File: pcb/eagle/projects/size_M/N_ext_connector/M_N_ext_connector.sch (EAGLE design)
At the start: 16 parts

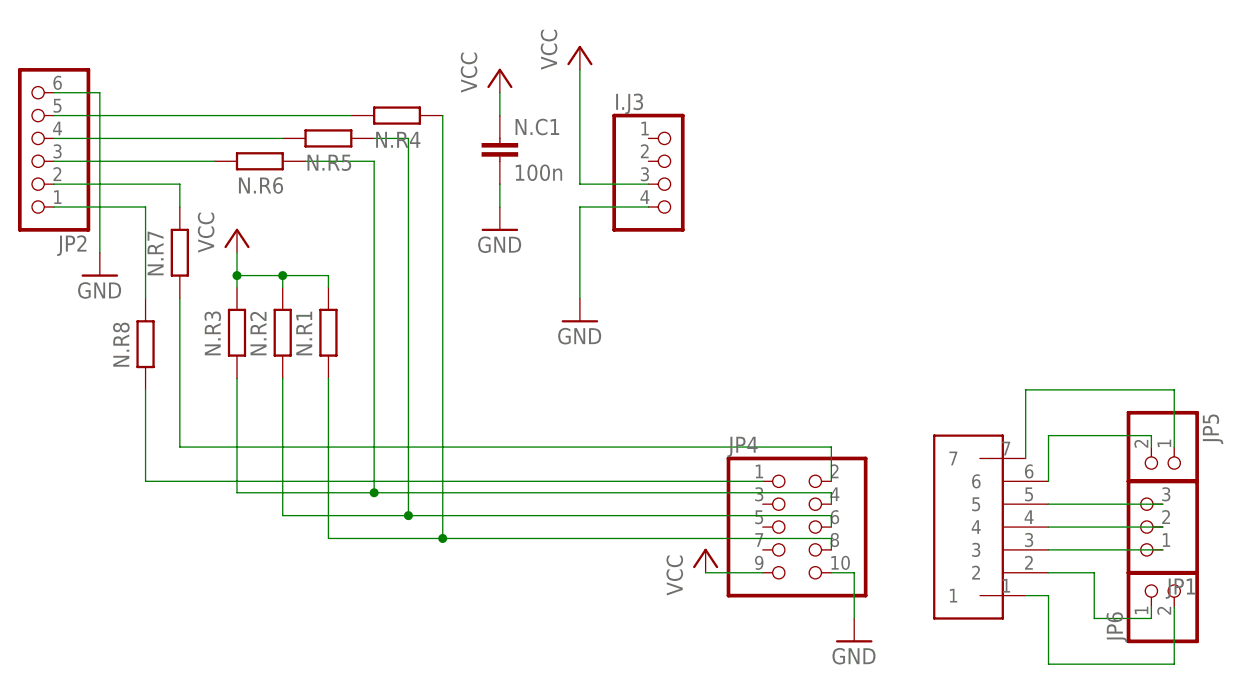
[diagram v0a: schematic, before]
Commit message: just adjustments
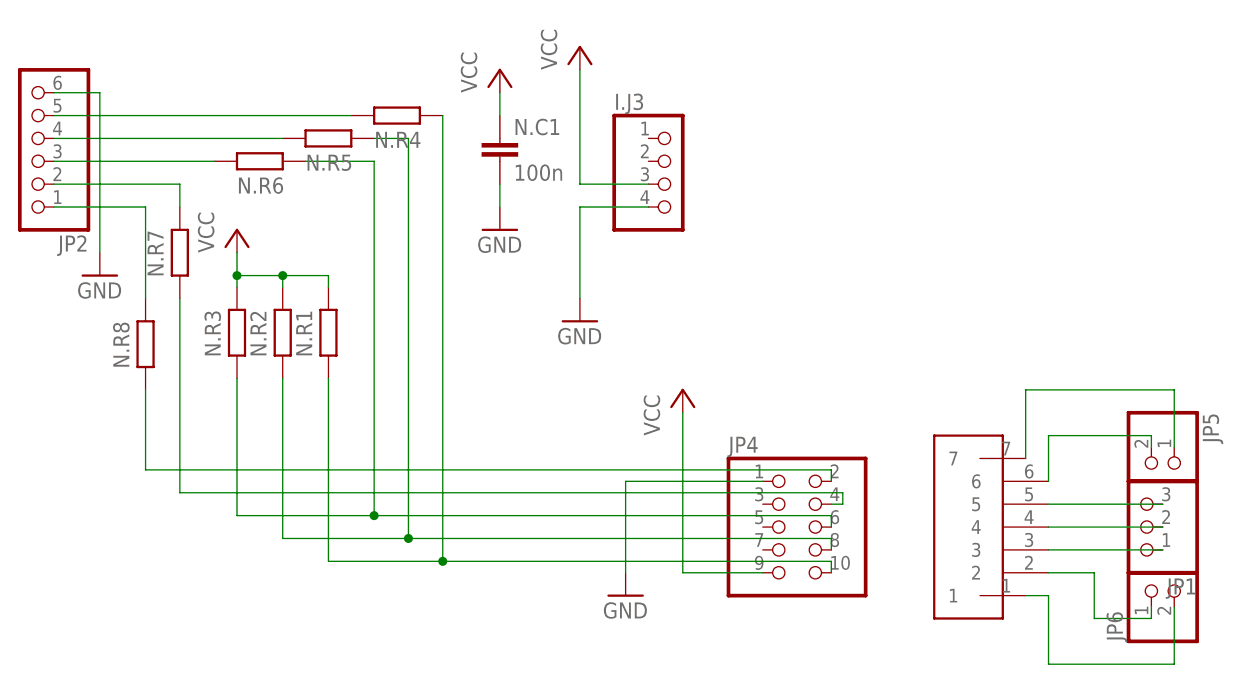
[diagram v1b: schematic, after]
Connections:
- net N$1 renamed PA6
- net N$12 renamed PA7
- net N$13 renamed SDA1
- net N$14 renamed PA3
- removed net N$15: JP6.2, U$1.1
- new net SCL1: JP5.2, U$1.6
- net GND: now also JP4.1; no longer JP4.10
- net GND1: now also JP5.1, U$1.7; no longer JP5.2, U$1.6
- net N$10: now also JP4.4; no longer JP4.2
- net N$11: now also JP4.2; no longer JP4.1
- net N$2: now also JP4.10; no longer JP4.8
- net N$3: now also JP4.8; no longer JP4.6
- net N$9: now also JP4.6; no longer JP4.4
- net VCC1: now also JP6.2, U$1.1; no longer JP5.1, U$1.7
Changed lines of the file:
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@@
 <attribute name="VALUE" x="111.76" y="20.32" size="1.778" layer="96"/>
 </instance>
-<instance part="GND4" gate="1" x="144.78" y="-12.7" smashed="yes">
-<attribute name="VALUE" x="142.24" y="-15.24" size="1.778" layer="96"/>
+<instance part="GND4" gate="1" x="119.38" y="-7.62" smashed="yes">
+<attribute name="VALUE" x="116.84" y="-10.16" size="1.778" layer="96"/>
 </instance>
 <instance part="GND5" gate="1" x="60.96" y="27.94" smashed="yes">
 <attribute name="VALUE" x="58.42" y="25.4" size="1.778" layer="96"/>
 </instance>
-<instance part="P+4" gate="VCC" x="128.27" y="-2.54" smashed="yes">
-<attribute name="VALUE" x="125.73" y="-7.62" size="1.778" layer="96" rot="R90"/>
+<instance part="P+4" gate="VCC" x="125.73" y="15.24" smashed="yes">
+<attribute name="VALUE" x="123.19" y="10.16" size="1.778" layer="96" rot="R90"/>
 </instance>
 <instance part="P+3" gate="VCC" x="76.2" y="33.02" smashed="yes">
@@
 <segment>
 <pinref part="GND4" gate="1" pin="GND"/>
-<wire x1="142.24" y1="-5.08" x2="144.78" y2="-5.08" width="0.1524" layer="91"/>
-<wire x1="144.78" y1="-5.08" x2="144.78" y2="-10.16" width="0.1524" layer="91"/>
-<pinref part="JP4" gate="A" pin="10"/>
+<pinref part="JP4" gate="A" pin="1"/>
+<wire x1="119.38" y1="-5.08" x2="119.38" y2="5.08" width="0.1524" layer="91"/>
+<wire x1="119.38" y1="5.08" x2="134.62" y2="5.08" width="0.1524" layer="91"/>
 </segment>
 </net>
@@
 <segment>
 <pinref part="P+4" gate="VCC" pin="VCC"/>
-<wire x1="128.27" y1="-5.08" x2="134.62" y2="-5.08" width="0.1524" layer="91"/>
 <pinref part="JP4" gate="A" pin="9"/>
+<wire x1="125.73" y1="12.7" x2="125.73" y2="-5.08" width="0.1524" layer="91"/>
+<wire x1="125.73" y1="-5.08" x2="134.62" y2="-5.08" width="0.1524" layer="91"/>
 </segment>
 </net>
 <net name="N$2" class="0">
 <segment>
-<wire x1="86.36" y1="-1.27" x2="99.06" y2="-1.27" width="0.1524" layer="91"/>
+<wire x1="86.36" y1="-3.81" x2="99.06" y2="-3.81" width="0.1524" layer="91"/>
 <pinref part="N.R1" gate="G$1" pin="2"/>
-<wire x1="86.36" y1="16.51" x2="86.36" y2="-1.27" width="0.1524" layer="91"/>
-<wire x1="99.06" y1="-1.27" x2="99.06" y2="45.72" width="0.1524" layer="91"/>
+<wire x1="86.36" y1="16.51" x2="86.36" y2="-3.81" width="0.1524" layer="91"/>
+<wire x1="99.06" y1="-3.81" x2="99.06" y2="45.72" width="0.1524" layer="91"/>
 <pinref part="N.R4" gate="G$1" pin="2"/>
+<wire x1="99.06" y1="-3.81" x2="142.24" y2="-3.81" width="0.1524" layer="91"/>
+<junction x="99.06" y="-3.81"/>
+<pinref part="JP4" gate="A" pin="10"/>
+<wire x1="142.24" y1="-5.08" x2="142.24" y2="-3.81" width="0.1524" layer="91"/>
+</segment>
+</net>
+<net name="N$3" class="0">
+<segment>
+<wire x1="81.28" y1="-1.27" x2="95.25" y2="-1.27" width="0.1524" layer="91"/>
+<pinref part="N.R2" gate="G$1" pin="2"/>
+<wire x1="81.28" y1="16.51" x2="81.28" y2="-1.27" width="0.1524" layer="91"/>
+<wire x1="91.44" y1="43.18" x2="95.25" y2="43.18" width="0.1524" layer="91"/>
+<wire x1="95.25" y1="43.18" x2="95.25" y2="-1.27" width="0.1524" layer="91"/>
+<pinref part="N.R5" gate="G$1" pin="2"/>
+<wire x1="95.25" y1="-1.27" x2="142.24" y2="-1.27" width="0.1524" layer="91"/>
+<junction x="95.25" y="-1.27"/>
 <pinref part="JP4" gate="A" pin="8"/>
-<wire x1="99.06" y1="-1.27" x2="142.24" y2="-1.27" width="0.1524" layer="91"/>
-<wire x1="142.24" y1="-1.27" x2="142.24" y2="-2.54" width="0.1524" layer="91"/>
-<junction x="99.06" y="-1.27"/>
-</segment>
-</net>
-<net name="N$3" class="0">
-<segment>
-<wire x1="81.28" y1="1.27" x2="95.25" y2="1.27" width="0.1524" layer="91"/>
-<pinref part="N.R2" gate="G$1" pin="2"/>
-<wire x1="81.28" y1="16.51" x2="81.28" y2="1.27" width="0.1524" layer="91"/>
-<wire x1="91.44" y1="43.18" x2="95.25" y2="43.18" width="0.1524" layer="91"/>
-<wire x1="95.25" y1="43.18" x2="95.25" y2="1.27" width="0.1524" layer="91"/>
-<pinref part="N.R5" gate="G$1" pin="2"/>
-<pinref part="JP4" gate="A" pin="6"/>
-<wire x1="95.25" y1="1.27" x2="142.24" y2="1.27" width="0.1524" layer="91"/>
-<wire x1="142.24" y1="1.27" x2="142.24" y2="0" width="0.1524" layer="91"/>
-<junction x="95.25" y="1.27"/>
+<wire x1="142.24" y1="-2.54" x2="142.24" y2="-1.27" width="0.1524" layer="91"/>
 </segment>
 </net>
 <net name="N$10" class="0">
 <segment>
-<wire x1="69.85" y1="25.4" x2="69.85" y2="8.89" width="0.1524" layer="91"/>
+<wire x1="69.85" y1="25.4" x2="69.85" y2="3.81" width="0.1524" layer="91"/>
 <pinref part="N.R7" gate="G$1" pin="2"/>
-<pinref part="JP4" gate="A" pin="2"/>
-<wire x1="142.24" y1="5.08" x2="142.24" y2="8.89" width="0.1524" layer="91"/>
-<wire x1="142.24" y1="8.89" x2="69.85" y2="8.89" width="0.1524" layer="91"/>
+<wire x1="143.51" y1="3.81" x2="69.85" y2="3.81" width="0.1524" layer="91"/>
+<pinref part="JP4" gate="A" pin="4"/>
+<wire x1="142.24" y1="2.54" x2="143.51" y2="2.54" width="0.1524" layer="91"/>
+<wire x1="143.51" y1="2.54" x2="143.51" y2="3.81" width="0.1524" layer="91"/>
 </segment>
 </net>
@@
 <net name="N$11" class="0">
 <segment>
-<pinref part="JP4" gate="A" pin="1"/>
-<wire x1="66.04" y1="15.24" x2="66.04" y2="5.08" width="0.1524" layer="91"/>
 <pinref part="N.R8" gate="G$1" pin="2"/>
-<wire x1="134.62" y1="5.08" x2="66.04" y2="5.08" width="0.1524" layer="91"/>
+<wire x1="66.04" y1="15.24" x2="66.04" y2="6.35" width="0.1524" layer="91"/>
+<pinref part="JP4" gate="A" pin="2"/>
+<wire x1="142.24" y1="5.08" x2="142.24" y2="6.35" width="0.1524" layer="91"/>
+<wire x1="142.24" y1="6.35" x2="66.04" y2="6.35" width="0.1524" layer="91"/>
 </segment>
 </net>
 <net name="N$9" class="0">
 <segment>
-<pinref part="JP4" gate="A" pin="4"/>
-<wire x1="142.24" y1="2.54" x2="142.24" y2="3.81" width="0.1524" layer="91"/>
-<wire x1="76.2" y1="3.81" x2="91.44" y2="3.81" width="0.1524" layer="91"/>
+<wire x1="76.2" y1="1.27" x2="91.44" y2="1.27" width="0.1524" layer="91"/>
 <pinref part="N.R3" gate="G$1" pin="2"/>
-<wire x1="76.2" y1="16.51" x2="76.2" y2="3.81" width="0.1524" layer="91"/>
+<wire x1="76.2" y1="16.51" x2="76.2" y2="1.27" width="0.1524" layer="91"/>
 <wire x1="83.82" y1="40.64" x2="91.44" y2="40.64" width="0.1524" layer="91"/>
-<wire x1="91.44" y1="40.64" x2="91.44" y2="3.81" width="0.1524" layer="91"/>
+<wire x1="91.44" y1="40.64" x2="91.44" y2="1.27" width="0.1524" layer="91"/>
 <pinref part="N.R6" gate="G$1" pin="2"/>
-<wire x1="142.24" y1="3.81" x2="91.44" y2="3.81" width="0.1524" layer="91"/>
-<junction x="91.44" y="3.81"/>
-</segment>
-</net>
-<net name="N$14" class="0">
+<wire x1="142.24" y1="1.27" x2="91.44" y2="1.27" width="0.1524" layer="91"/>
+<junction x="91.44" y="1.27"/>
+<pinref part="JP4" gate="A" pin="6"/>
+<wire x1="142.24" y1="0" x2="142.24" y2="1.27" width="0.1524" layer="91"/>
+</segment>
+</net>
+<net name="PA3" class="0">
 <segment>
 <pinref part="U$1" gate="G$1" pin="2"/>
@@
 </segment>
 </net>
-<net name="N$15" class="0">
+<net name="VCC1" class="0">
 <segment>
 <pinref part="U$1" gate="G$1" pin="1"/>
@@
 </segment>
 </net>
-<net name="N$12" class="0">
+<net name="PA7" class="0">
 <segment>
 <pinref part="U$1" gate="G$1" pin="4"/>
@@
 </segment>
 </net>
-<net name="N$13" class="0">
+<net name="SDA1" class="0">
 <segment>
 <pinref part="JP1" gate="A" pin="3"/>
@@
 </segment>
 </net>
-<net name="GND1" class="0">
+<net name="SCL1" class="0">
 <segment>
 <pinref part="U$1" gate="G$1" pin="6"/>
@@
 </segment>
 </net>
-<net name="VCC1" class="0">
+<net name="GND1" class="0">
 <segment>
 <pinref part="U$1" gate="G$1" pin="7"/>
@@
 </segment>
 </net>
-<net name="N$1" class="0">
+<net name="PA6" class="0">
 <segment>
 <pinref part="U$1" gate="G$1" pin="3"/>
